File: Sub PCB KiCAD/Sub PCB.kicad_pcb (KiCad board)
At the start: 2 copper layers, 12 parts

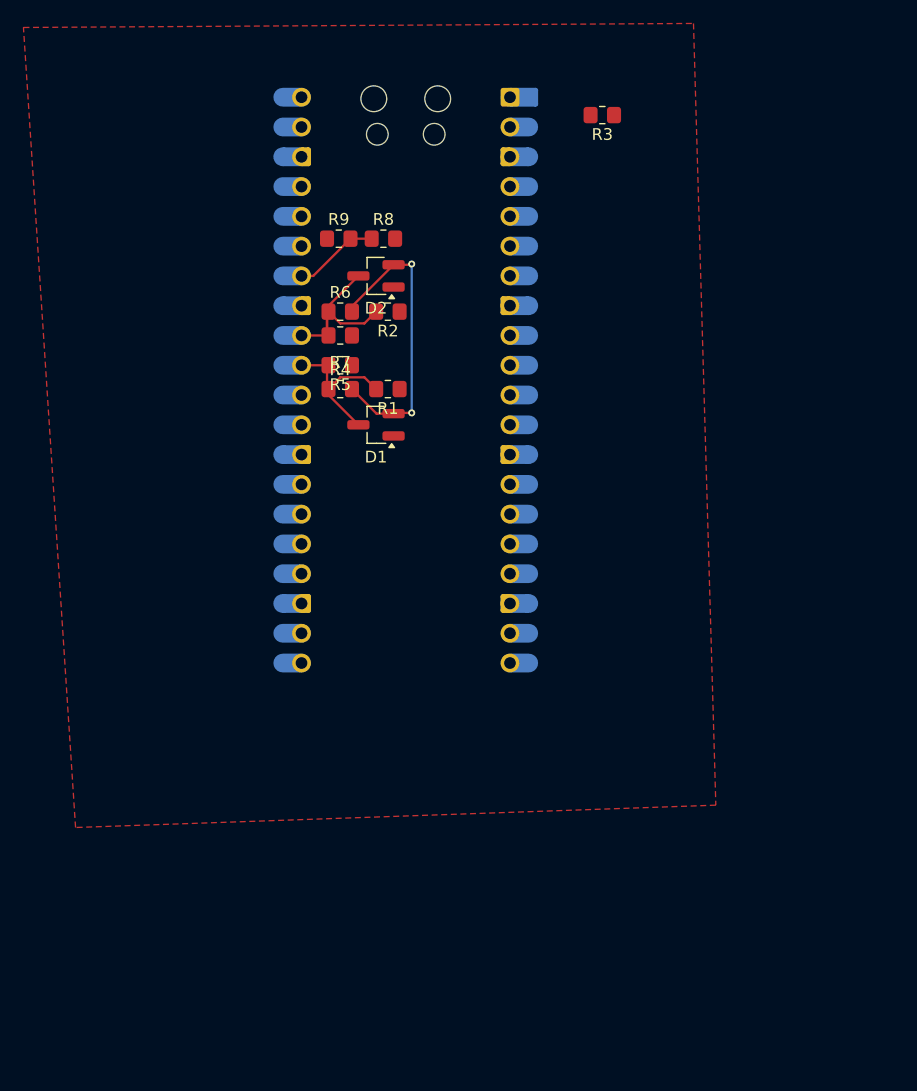
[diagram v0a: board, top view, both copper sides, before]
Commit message: .
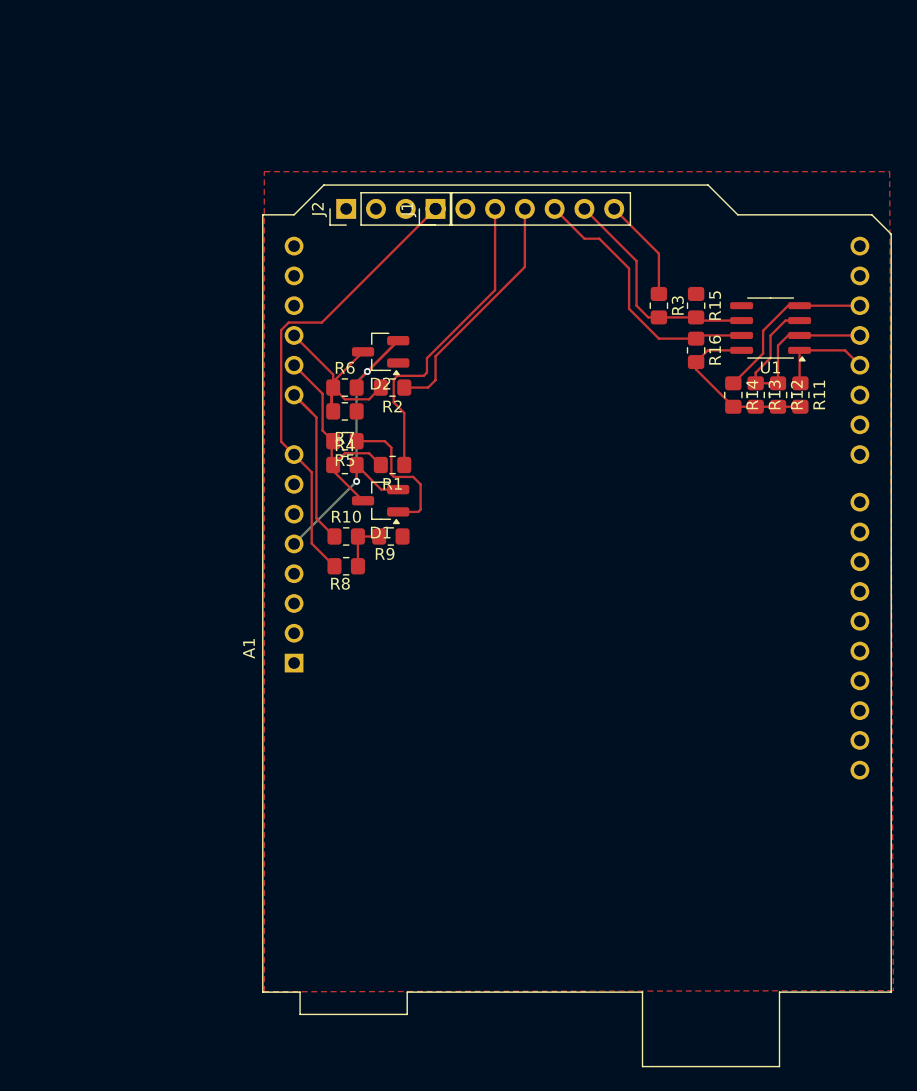
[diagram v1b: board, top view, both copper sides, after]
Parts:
- added J1: ~, Connector_PinHeader_2.54mm:PinHeader_1x07_P2.54mm_Vertical, F.Cu at (157.5, 67.9)
- added J2: ~, Connector_PinHeader_2.54mm:PinHeader_1x04_P2.54mm_Vertical, F.Cu at (149.9, 67.9)
- added R10: 10k, Resistor_SMD:R_0805_2012Metric_Pad1.20x1.40mm_HandSolder, F.Cu at (149.9, 95.9)
- added R11: 10k, Resistor_SMD:R_0805_2012Metric_Pad1.20x1.40mm_HandSolder, F.Cu at (188.6, 83.8)
- added R12: 10k, Resistor_SMD:R_0805_2012Metric_Pad1.20x1.40mm_HandSolder, F.Cu at (186.7, 83.8)
- added R13: 10k, Resistor_SMD:R_0805_2012Metric_Pad1.20x1.40mm_HandSolder, F.Cu at (184.8, 83.8)
- added R14: 10k, Resistor_SMD:R_0805_2012Metric_Pad1.20x1.40mm_HandSolder, F.Cu at (182.9, 83.8)
- added R15: 20k, Resistor_SMD:R_0805_2012Metric_Pad1.20x1.40mm_HandSolder, F.Cu at (179.7, 76.2)
- added R16: 20k, Resistor_SMD:R_0805_2012Metric_Pad1.20x1.40mm_HandSolder, F.Cu at (179.7, 80.0)
- added U1: MAX485E, Package_SO:SOIC-8_3.9x4.9mm_P1.27mm, F.Cu at (186.1, 78.1)
- A1: value RaspberryPi_Pico -> Arduino_UNO_R3; footprint Module:RaspberryPi_Pico_Common_Unspecified -> Module:Arduino_UNO_R3; moved to F.Cu
- moved R8 28.1 mm to (149.9, 98.4), turned to 180 degrees
- moved A1 25.9 mm to (145.4, 106.7), turned to 90 degrees
- moved R9 25.8 mm to (153.7, 95.9), turned to 180 degrees
- moved R3 17.0 mm to (176.5, 76.2), turned to -90 degrees
- moved D1 6.49 mm to (152.8, 92.8)
- moved D2 6.49 mm to (152.8, 80.1)
- moved R1 6.49 mm to (153.8, 89.8)
- moved R2 6.49 mm to (153.8, 83.2)
- moved R4 6.49 mm to (149.8, 89.8)
- moved R5 6.49 mm to (149.8, 87.8)
- moved R6 6.49 mm to (149.8, 83.2)
- moved R7 6.49 mm to (149.8, 85.2)
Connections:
- A1 pad 1: /UART0_TX -> unconnected-(A1-NC-Pad1)
- A1 pad 10: unconnected-(A1-GPIO7-Pad10) -> /ADDR_1
- A1 pad 11: unconnected-(A1-GPIO8-Pad11) -> /ADDR_2
- A1 pad 13: GND -> /I2C_SDA
- A1 pad 14: unconnected-(A1-GPIO10-Pad14) -> /I2C_SCL
- A1 pad 15: unconnected-(A1-GPIO11-Pad15) -> /UART0_TX
- A1 pad 16: unconnected-(A1-GPIO12-Pad16) -> /UART0_RX
- A1 pad 17: unconnected-(A1-GPIO13-Pad17) -> /UART1_TX
- A1 pad 18: GND -> /UART1_TX_EN
- A1 pad 19: unconnected-(A1-GPIO14-Pad19) -> /UART1_RX
- A1 pad 2: /UART0_RX -> unconnected-(A1-IOREF-Pad2)
- A1 pad 23: GND -> unconnected-(A1-D8-Pad23)
- A1 pad 28: GND -> unconnected-(A1-D13-Pad28)
- A1 pad 29: unconnected-(A1-GPIO22-Pad29) -> GND
- A1 pad 3: GND -> unconnected-(A1-~{RESET}-Pad3)
- A1 pad 31: /ADDR_1 -> unconnected-(A1-SDA/A4-Pad31)
- A1 pad 32: /ADDR_2 -> unconnected-(A1-SCL/A5-Pad32)
- A1 pad 5: unconnected-(A1-GPIO3-Pad5) -> +5V
- A1 pad 6: /UART1_TX -> GND
- A1 pad 7: /UART1_RX -> GND
- A1 pad 8: GND -> +12V
- A1 pad 9: unconnected-(A1-GPIO6-Pad9) -> /V_Supply
- D1 pad 2: +3V3 -> +5V
- D2 pad 2: +3V3 -> +5V
- R4 pad 2: +3V3 -> +5V
- R6 pad 2: +3V3 -> +5V
- R8 pad 1: /V_Supply -> Net-(R10-Pad2)
- R9 pad 2: /V_Supply -> Net-(R10-Pad2)
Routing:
- net +5V: track 0.00 -> 47.6 mm, vias 0 -> 2
- net +12V: track 0.00 -> 40.1 mm
- net Net-(J1-Pin_3): track 0.00 -> 27.1 mm
- net +3V3: track 26.1 -> 0.00 mm, vias 2 -> 0
- net /RS485_B: track 0.00 -> 22.7 mm
- net Net-(J1-Pin_4): track 0.00 -> 20.7 mm
- net /UART1_TX_EN: track 0.00 -> 20.1 mm
- net /RS485_A: track 0.00 -> 19.6 mm
- net /UART1_TX: track 0.00 -> 14.7 mm
- net GND: track 0.00 -> 12.5 mm
- net Net-(J1-Pin_7): track 0.00 -> 8.83 mm
- net /UART1_RX: track 0.00 -> 8.51 mm
- net /V_Supply: track 7.30 -> 15.6 mm
- net /ADDR_1: track 13.4 -> 19.0 mm
- net Net-(R10-Pad2): track 0.00 -> 4.51 mm
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
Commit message: .
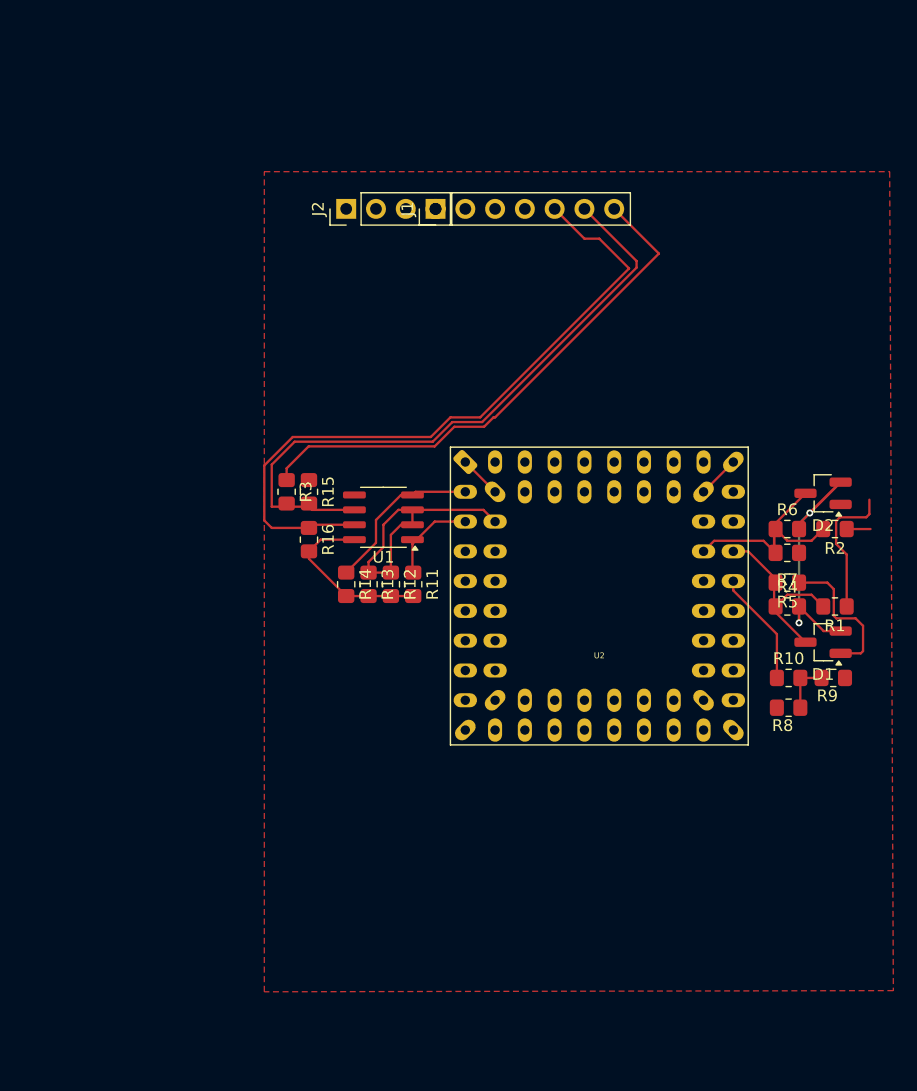
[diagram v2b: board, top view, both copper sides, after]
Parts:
- removed A1: Arduino_UNO_R3, Module:Arduino_UNO_R3
- added U2: Pimoroni PGA2350, Skippy's:PGA2350, F.Cu at (171.4, 101.0)
- moved R1 39.6 mm to (191.5, 101.9)
- moved R2 39.6 mm to (191.5, 95.2)
- moved R4 39.6 mm to (187.5, 101.9)
- moved R5 39.6 mm to (187.5, 99.8)
- moved R6 39.6 mm to (187.5, 95.2)
- moved R7 39.6 mm to (187.5, 97.3)
- moved R9 39.6 mm to (191.4, 108.0)
- moved D1 39.6 mm to (190.5, 104.9)
- moved D2 39.6 mm to (190.5, 92.2)
- moved R10 39.6 mm to (187.6, 108.0)
- moved R8 39.6 mm to (187.6, 110.5)
- moved R11 36.8 mm to (155.6, 100.0)
- moved R12 36.8 mm to (153.7, 100.0)
- moved R13 36.8 mm to (151.8, 100.0)
- moved R16 36.8 mm to (146.7, 96.2)
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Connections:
- net +5V renamed +3V3
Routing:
- net +12V: track 40.1 -> 0.00 mm
- net Net-(J1-Pin_7): track 8.83 -> 45.7 mm
- net /RS485_B: track 22.7 -> 59.3 mm
- net /RS485_A: track 19.6 -> 55.7 mm
- net Net-(J1-Pin_4): track 20.7 -> 2.03 mm
- net Net-(J1-Pin_3): track 27.1 -> 12.0 mm
- net +3V3: track 47.6 -> 40.1 mm
- net GND: track 12.5 -> 19.7 mm
- net /V_Supply: track 15.6 -> 9.79 mm
- net /UART1_TX_EN: track 20.1 -> 23.7 mm
- net /ADDR_1: track 19.0 -> 16.1 mm
- net /ADDR_2: track 18.5 -> 20.3 mm
- net /UART1_TX: track 14.7 -> 14.2 mm
